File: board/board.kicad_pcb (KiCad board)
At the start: 2 copper layers, 21 x 13 mm, 1 part

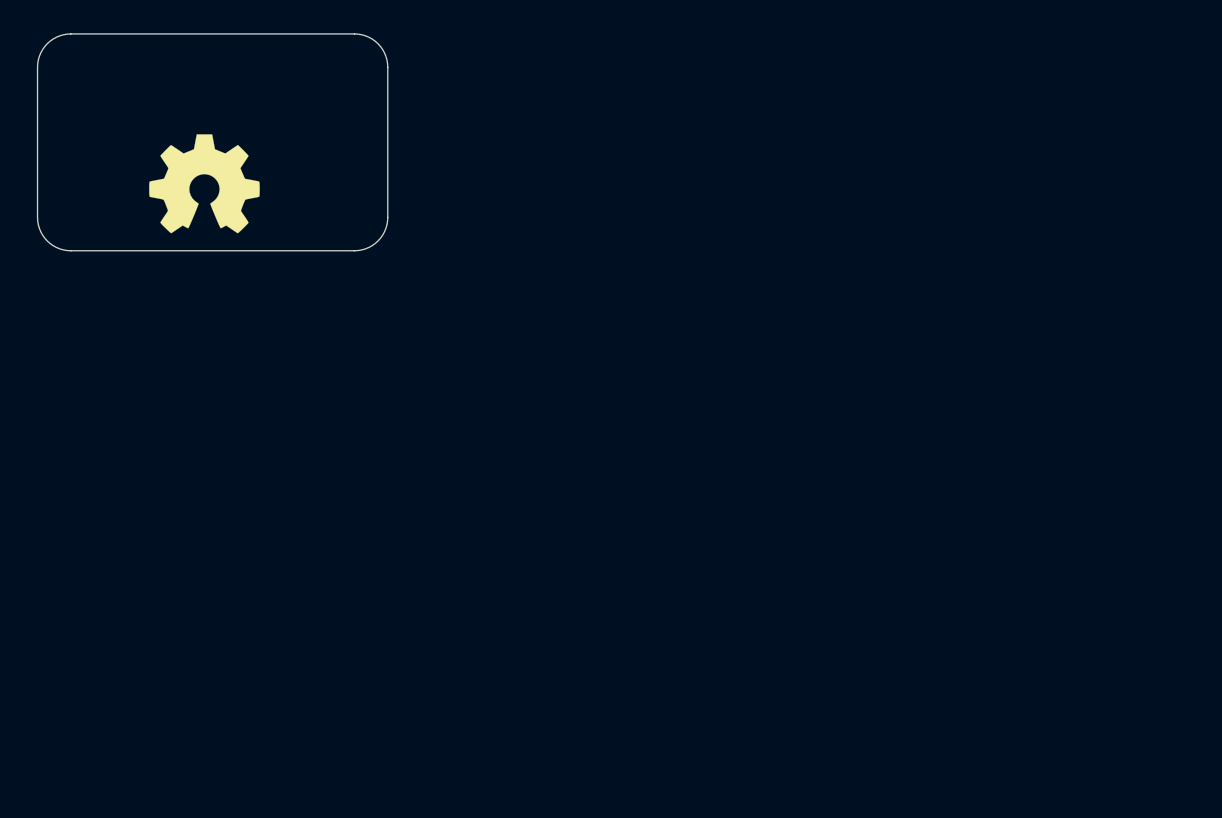
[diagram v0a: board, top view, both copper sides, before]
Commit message: initial
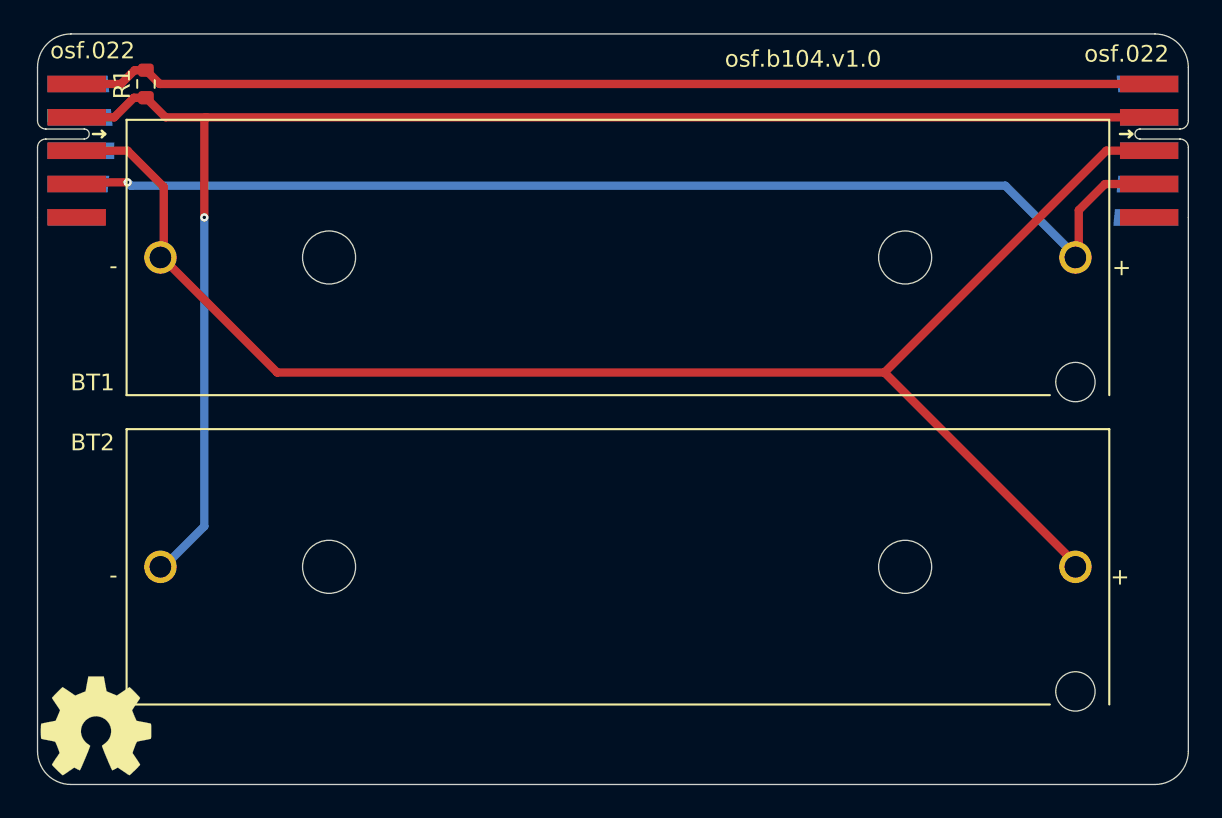
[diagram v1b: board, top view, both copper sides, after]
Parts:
- added BT1: BHAA-3-G, b104:BAT_BHAA-3-G, F.Cu at (174.8, 103.4)
- added BT2: BHAA-3-G, b104:BAT_BHAA-3-G, F.Cu at (174.8, 122.0)
- added J1: 022_battery_cells, on_edge:on_edge_2x05_device, F.Cu at (140.0, 97.0)
- added J2: 022_battery_cells, on_edge:on_edge_2x05_host, F.Cu at (209.0, 97.0)
- added R1: 0R, Resistor_SMD:R_0603_1608Metric, F.Cu at (146.5, 93.0)
- moved LOGO1 33.1 mm to (143.5, 131.5)
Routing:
- net /implementation/C1+C2-: track 0.00 -> 94.3 mm
- net /implementation/C1-: track 0.00 -> 93.3 mm, vias 0 -> 1
- net /implementation/C2+: track 0.00 -> 69.8 mm, vias 0 -> 1
- net GND: track 0.00 -> 65.0 mm
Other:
- board size 21 x 13 mm -> 69 x 45 mm
- board text added: "osf.022"
- board text added: "osf.b104.v1.0"
